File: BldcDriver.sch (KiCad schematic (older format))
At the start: 54 parts, among them J1 Motor Out, J2 DC Jack, J3 STM32_Debug_5pin, Q1 2SK4033, Q2 2SK4033, Q3 2SK4033, Q4 2SK4033, Q5 2SK4033, Q6 2SK4033, U1 IR2101, U2 IR2101, U3 IR2101, U4 NJM78L33SU3, U5 STM32F303K8Tx, X1 12MHz

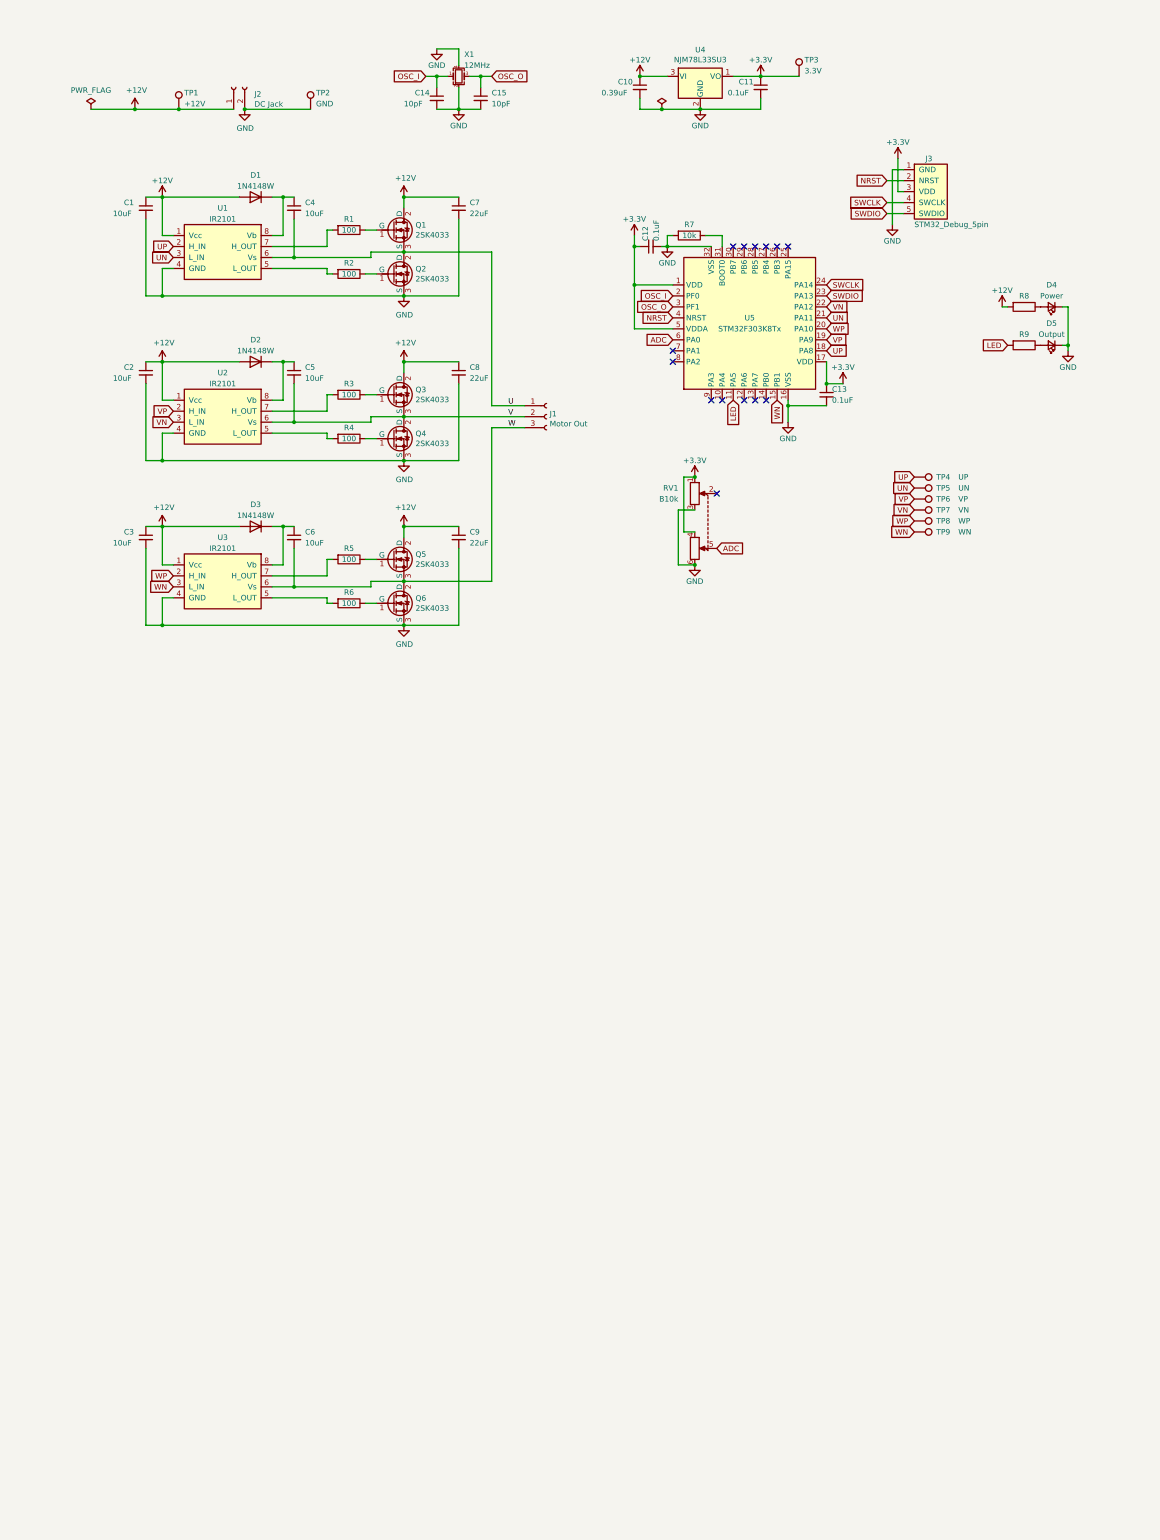
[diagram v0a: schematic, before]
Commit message: 基板 V4.0
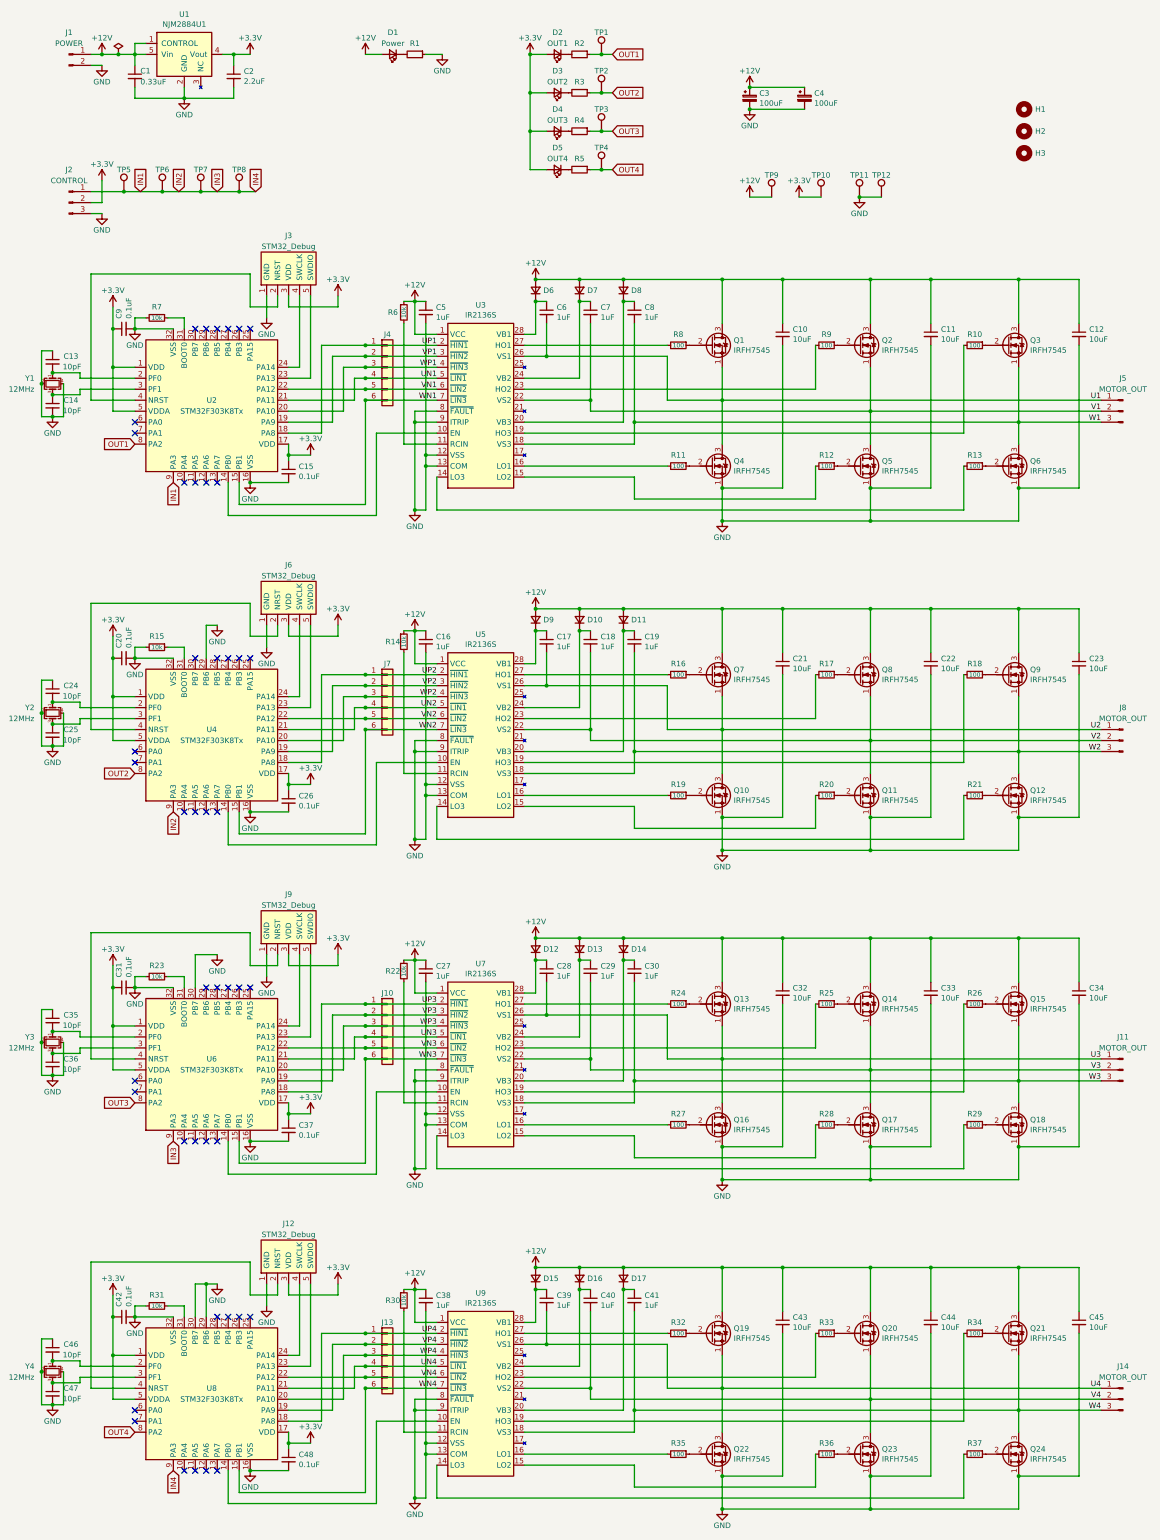
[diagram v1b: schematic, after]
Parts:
- removed C3, C4: 10uF, Capacitor_SMD:C_0603_1608Metric_Pad1.05x0.95mm_HandSolder, symbol Device:C_Small
- removed D1, D2, D3: 1N4148W, Diode_SMD:D_SOD-123, symbol Device:D
- removed J1: Motor Out, Connector_PinSocket_2.54mm:PinSocket_1x03_P2.54mm_Vertical, symbol Connector:Conn_01x03_Female
- removed J2: DC Jack, Connector_PinSocket_2.54mm:PinSocket_1x02_P2.54mm_Vertical, symbol Connector:Conn_01x02_Female
- removed Q1, Q2, Q3, Q4, Q5, Q6: 2SK4033, Package_TO_SOT_THT:TO-220-3_Vertical, symbol BldcDriver:2SK4017
- removed R1, R2, R3, R4, R5, R6: 100, Resistor_SMD:R_0603_1608Metric_Pad1.05x0.95mm_HandSolder, symbol Device:R
- removed R7: 10k, Resistor_SMD:R_0603_1608Metric_Pad1.05x0.95mm_HandSolder, symbol Device:R
- removed R8, R9: R, Resistor_SMD:R_0603_1608Metric_Pad1.05x0.95mm_HandSolder, symbol Device:R
- removed RV1: B10k, Potentiometer_THT:Potentiometer_Alps_RK097_Dual_Horizontal, symbol Device:R_POT_Dual
- removed U1, U2, U3: IR2101, BldcDriver:SOIC-8_3.9x4.9mm_P1.27mm, symbol BldcDriver:IR2101
- removed U4: NJM78L33SU3, Package_TO_SOT_SMD:SOT-89-3, symbol BldcDriver:NJM78L33SU3
- removed U5: STM32F303K8Tx, BldcDriver:LQFP-32_7x7mm_P0.8mm_FusionPCB, symbol BldcDriver:STM32F303K8Tx
- removed X1: 12MHz, BldcDriver:Crystal_SMD_3225-4Pin_3.2x2.5mm_HandSoldering, symbol Device:Crystal_GND24_Small
- added C16, C17, C18, C19, C27, C28, C29, C30, C38, C39, C40, C41: 1uF, BldcDriver:1608Metric, symbol Device:C_Small
- added C20, C26, C31, C37, C42, C48: 0.1uF, BldcDriver:1608Metric, symbol Device:C_Small
- added C21, C22, C23, C32, C33, C34, C43, C44, C45: 10uF, BldcDriver:1608Metric, symbol Device:C_Small
- added C24, C25, C35, C36, C46, C47: 10pF, BldcDriver:1005Metric, symbol Device:C_Small
- added C3, C4: 100uF, BldcDriver:CP_Elec_6.3x7.7, symbol Device:CP_Small
- added D1: Power, BldcDriver:1608Metric, symbol Device:LED_Small
- added D10, D11, D12, D13, D14, D15, D16, D17, D6, D7, D8, D9: 1N4148W, BldcDriver:D_SOD-123, symbol Device:D_Small
- added D2: OUT1, BldcDriver:1608Metric, symbol Device:LED_Small
- added D3: OUT2, BldcDriver:1608Metric, symbol Device:LED_Small
- added H1: MountingHole, BldcDriver:MountingHole_4.3mm_M4, symbol Mechanical:MountingHole
- added H2, H3: MountingHole, BldcDriver:MountingHole_2mm, symbol Mechanical:MountingHole
- added J1: POWER, BldcDriver:JST_XH_S2B-XH-A_1x02_P2.50mm_Horizontal, symbol Connector:Conn_01x02_Male
- added J10, J13, J4, J7: Conn_01x06, BldcDriver:Pin_1x06_P2.54mm, symbol Connector_Generic:Conn_01x06
- added J11, J14, J5, J8: MOTOR_OUT, BldcDriver:JST_XH_S3B-XH-A_1x03_P2.50mm_Horizontal, symbol Connector:Conn_01x03_Male
- added J12, J6, J9: STM32_Debug, BldcDriver:STM32_Debug_5pin, symbol BldcDriver:STM32_Debug_5pin
- added J2: CONTROL, BldcDriver:JST_XH_S3B-XH-A_1x03_P2.50mm_Horizontal, symbol Connector:Conn_01x03_Male
- added Q1, Q10, Q11, Q12, Q13, Q14, Q15, Q16, Q17, Q18, Q19, Q2, Q20, Q21, Q22, Q23, Q24, Q3, Q4, Q5, Q6, Q7, Q8, Q9: IRFH7545, BldcDriver:VSONP-8-1EP_5x6_P1.27mm, symbol Device:Q_NMOS_SGD
- added R1, R2, R3, R4, R5: R, BldcDriver:1608Metric, symbol Device:R_Small
- added R10, R11, R12, R13, R16, R17, R18, R19, R20, R21, R24, R25, R26, R27, R28, R29, R32, R33, R34, R35, R36, R37, R8, R9: 100, BldcDriver:1608Metric, symbol Device:R_Small
- added R14, R15, R22, R23, R30, R31, R6, R7: 10k, BldcDriver:1608Metric, symbol Device:R_Small
- added TP10, TP11, TP12: TestPoint, BldcDriver:TestPoint_THTPad_D1.3mm_Drill0.9mm, symbol Connector:TestPoint
- added U1: NJM2884U1, BldcDriver:SOT-89-5, symbol BldcDriver:NJM2884U1
- added U2, U4, U6, U8: STM32F303K8Tx, BldcDriver:LQFP-32_7x7mm_P0.8mm_FusionPCB, symbol BldcDriver:STM32F303K8Tx
- added U3, U5, U7, U9: IR2136S, BldcDriver:SOIC-28W_7.5x17.9mm_P1.27mm, symbol BldcDriver:IR2136S
- added Y1, Y2, Y3, Y4: 12MHz, BldcDriver:Crystal_SMD_3225-4Pin_3.2x2.5mm_HandSoldering, symbol Device:Crystal_GND24_Small
- C1: value 10uF -> 0.33uF; footprint Capacitor_SMD:C_0603_1608Metric_Pad1.05x0.95mm_HandSolder -> BldcDriver:1608Metric
- C10: value 0.39uF -> 10uF; footprint Capacitor_SMD:C_0603_1608Metric_Pad1.05x0.95mm_HandSolder -> BldcDriver:1608Metric
- C11, C12: value 0.1uF -> 10uF; footprint Capacitor_SMD:C_0603_1608Metric_Pad1.05x0.95mm_HandSolder -> BldcDriver:1608Metric
- C13: value 0.1uF -> 10pF; footprint Capacitor_SMD:C_0603_1608Metric_Pad1.05x0.95mm_HandSolder -> BldcDriver:1005Metric
- C14: footprint BldcDriver:C_0402_1005Metric -> BldcDriver:1005Metric
- C15: value 10pF -> 0.1uF; footprint BldcDriver:C_0402_1005Metric -> BldcDriver:1608Metric
- C2: value 10uF -> 2.2uF; footprint Capacitor_SMD:C_0603_1608Metric_Pad1.05x0.95mm_HandSolder -> BldcDriver:1608Metric
- C5, C6: value 10uF -> 1uF; footprint Capacitor_SMD:C_0603_1608Metric_Pad1.05x0.95mm_HandSolder -> BldcDriver:1608Metric
- C7, C8: value 22uF -> 1uF; footprint Capacitor_SMD:C_1210_3225Metric_Pad1.42x2.65mm_HandSolder -> BldcDriver:1608Metric
- C9: value 22uF -> 0.1uF; footprint Capacitor_SMD:C_1210_3225Metric_Pad1.42x2.65mm_HandSolder -> BldcDriver:1608Metric
- D4: value Power -> OUT3; footprint LED_SMD:LED_0603_1608Metric_Pad1.05x0.95mm_HandSolder -> BldcDriver:1608Metric
- D5: value Output -> OUT4; footprint LED_SMD:LED_0603_1608Metric_Pad1.05x0.95mm_HandSolder -> BldcDriver:1608Metric
- J3: value STM32_Debug_5pin -> STM32_Debug
- TP1: value +12V -> TestPoint; footprint BldcDriver:TestPoint_THTPad_D2.0mm_Drill1.0mm -> BldcDriver:TestPoint_THTPad_D1.3mm_Drill0.9mm
- TP2: value GND -> TestPoint; footprint BldcDriver:TestPoint_THTPad_D2.0mm_Drill1.0mm -> BldcDriver:TestPoint_THTPad_D1.3mm_Drill0.9mm
- TP3: value 3.3V -> TestPoint; footprint BldcDriver:TestPoint_THTPad_D2.0mm_Drill1.0mm -> BldcDriver:TestPoint_THTPad_D1.3mm_Drill0.9mm
- TP4: value UP -> TestPoint; footprint BldcDriver:TestPoint_THTPad_D2.0mm_Drill1.0mm -> BldcDriver:TestPoint_THTPad_D1.3mm_Drill0.9mm
- TP5: value UN -> TestPoint; footprint BldcDriver:TestPoint_THTPad_D2.0mm_Drill1.0mm -> BldcDriver:TestPoint_THTPad_D1.3mm_Drill0.9mm
- TP6: value VP -> TestPoint; footprint BldcDriver:TestPoint_THTPad_D2.0mm_Drill1.0mm -> BldcDriver:TestPoint_THTPad_D1.3mm_Drill0.9mm
- TP7: value VN -> TestPoint; footprint BldcDriver:TestPoint_THTPad_D2.0mm_Drill1.0mm -> BldcDriver:TestPoint_THTPad_D1.3mm_Drill0.9mm
- TP8: value WP -> TestPoint; footprint BldcDriver:TestPoint_THTPad_D2.0mm_Drill1.0mm -> BldcDriver:TestPoint_THTPad_D1.3mm_Drill0.9mm
- TP9: value WN -> TestPoint; footprint BldcDriver:TestPoint_THTPad_D2.0mm_Drill1.0mm -> BldcDriver:TestPoint_THTPad_D1.3mm_Drill0.9mm
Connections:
- net OSC_O is gone; now on net +3V3: C15.1
- net V is gone; now on net GND: C5.2
- net VN is gone; now on net IN1: TP7.1
- net VP is gone; now on net IN1: TP6.1
- net WN is gone; now on net +12V: TP9.1
- net WP is gone; now on net IN1: TP8.1
- net +12V: now also C11.1, C12.1, C5.1, C16.1, C21.1, C22.1, C23.1, C27.1, C3.1, C32.1, C33.1, C34.1, C38.1, C4.1, C43.1, C44.1, C45.1, D1.2 (A), D10.2 (A), D11.2 (A), D12.2 (A), D13.2 (A), D14.2 (A), D15.2 (A), D16.2 (A), D17.2 (A), D6.2 (A), D7.2 (A), D8.2 (A), D9.2 (A), J1.1 (Pin_1), Q1.3 (D), Q13.3 (D), Q14.3 (D), Q15.3 (D), Q19.3 (D), Q2.3 (D), Q20.3 (D), Q21.3 (D), Q3.3 (D), Q7.3 (D), Q8.3 (D), Q9.3 (D), R14.1, R22.1, R30.1, R6.1, U1.1 (CONTROL), U1.5 (Vin), U3.1 (VCC), U5.1 (VCC), U7.1 (VCC), U9.1 (VCC); no longer C2.1, C7.1, C8.1, C9.1, TP1.1
- net +3V3: now also C2.1, C9.1, D4.2 (A), D5.2 (A), C20.1, C26.1, C31.1, C37.1, C42.1, C48.1, D2.2 (A), D3.2 (A), J12.3 (VDD), J2.2 (Pin_2), J6.3 (VDD), J9.3 (VDD), TP10.1, U1.4 (Vout), U2.1 (VDD), U2.17 (VDD), U2.5 (VDDA), U4.1 (VDD), U4.17 (VDD), U4.5 (VDDA), U6.1 (VDD), U6.17 (VDD), U6.5 (VDDA), U8.1 (VDD), U8.17 (VDD), U8.5 (VDDA); no longer C11.1, C12.1, C13.1, TP3.1
- net GND: now also C13.1, C16.2, C20.2, C21.2, C22.2, C23.2, C24.1, C25.2, C26.2, C27.2, C3.2, C31.2, C32.2, C33.2, C34.2, C35.1, C36.2, C37.2, C38.2, C4.2, C42.2, C43.2, C44.2, C45.2, C46.1, C47.2, C48.2, J1.2 (Pin_2), J12.1 (GND), J2.3 (Pin_3), J6.1 (GND), J9.1 (GND), Q10.1 (S), Q11.1 (S), Q12.1 (S), Q16.1 (S), Q17.1 (S), Q18.1 (S), Q22.1 (S), Q23.1 (S), Q24.1 (S), Q4.1 (S), Q5.1 (S), Q6.1 (S), R1.1, R15.2, R23.2, R31.2, R7.2, TP11.1, TP12.1, U1.2 (GND), U2.16 (VSS), U2.32 (VSS), U3.12 (VSS), U3.13 (COM), U3.8 (~FAULT), U3.9 (ITRIP), U4.16 (VSS), U4.29 (PB6), U4.32 (VSS), U5.12 (VSS), U5.13 (COM), U5.8 (~FAULT), U5.9 (ITRIP), U6.16 (VSS), U6.30 (PB7), U6.32 (VSS), U7.12 (VSS), U7.13 (COM), U7.8 (~FAULT), U7.9 (ITRIP), U8.16 (VSS), U8.29 (PB6), U8.30 (PB7), U8.32 (VSS), U9.12 (VSS), U9.13 (COM), U9.8 (~FAULT), U9.9 (ITRIP), Y1.2, Y1.4, Y2.2, Y2.4, Y3.2, Y3.4, Y4.2, Y4.4; no longer C13.2, C7.2, C8.2, D4.1 (K), D5.1 (K), TP2.1
- net at C6.1: now also D6.1 (K), U3.28 (VB1)
- net NRST: no longer names the net of J3.2 (NRST)
- net NRST: now also U2.4 (NRST)
- net OSC_I: no longer names the net of C14.1
- net OSC_I: now also U2.3 (PF1), Y1.3
- net SWCLK: no longer names the net of J3.4 (SWCLK)
- net SWCLK: now also U2.24 (PA14)
- net SWDIO: no longer names the net of J3.5 (SWDIO)
- net SWDIO: now also U2.23 (PA13)
- net UN renamed IN1
- net IN1: now also J2.1 (Pin_1), U2.9 (PA3), U4.9 (PA3), U6.9 (PA3), U8.9 (PA3)
- net UP renamed OUT4
- net OUT4: now also R5.1, U8.8 (PA2)
- net W renamed U1
- net U1: now also J5.1 (Pin_1), Q1.1 (S), Q4.3 (D), U3.26 (VS1)
- new net: U2.14 (PB0), U3.10 (EN)
- new net: R6.2, U3.11 (RCIN)
- new net: R13.2, U3.14 (LO3)
- new net: R12.2, U3.15 (LO2)
- new net: R11.2, U3.16 (LO1)
- new net: R10.2, U3.19 (HO3)
- new net: C8.1, D8.1 (K), U3.20 (VB3)
- new net: R9.2, U3.23 (HO2)
- new net: C7.1, D7.1 (K), U3.24 (VB2)
- new net: R8.2, U3.27 (HO1)
- new net: C13.2, U2.2 (PF0), Y1.1
- new net: R7.1, U2.31 (BOOT0)
- new net: Q1.2 (G), R8.1
- new net: Q4.2 (G), R11.1
- new net: Q2.2 (G), R9.1
- new net: Q5.2 (G), R12.1
- new net: Q3.2 (G), R10.1
- new net: Q6.2 (G), R13.1
- new net: U4.14 (PB0), U5.10 (EN)
- new net: R14.2, U5.11 (RCIN)
- new net: R21.2, U5.14 (LO3)
- new net: R20.2, U5.15 (LO2)
- new net: R19.2, U5.16 (LO1)
- new net: R18.2, U5.19 (HO3)
- new net: C19.1, D11.1 (K), U5.20 (VB3)
- new net: R17.2, U5.23 (HO2)
- new net: C18.1, D10.1 (K), U5.24 (VB2)
- new net: R16.2, U5.27 (HO1)
- new net: C17.1, D9.1 (K), U5.28 (VB1)
- new net: C24.2, U4.2 (PF0), Y2.1
- new net: J6.5 (SWDIO), U4.23 (PA13)
- new net: J6.4 (SWCLK), U4.24 (PA14)
- new net: C25.1, U4.3 (PF1), Y2.3
- new net: R15.1, U4.31 (BOOT0)
- new net: J6.2 (NRST), U4.4 (NRST)
- new net: Q7.2 (G), R16.1
- new net: Q10.2 (G), R19.1
- new net: Q8.2 (G), R17.1
- new net: Q11.2 (G), R20.1
- new net: Q9.2 (G), R18.1
- new net: Q12.2 (G), R21.1
- new net: U6.14 (PB0), U7.10 (EN)
- new net: R22.2, U7.11 (RCIN)
- new net: R29.2, U7.14 (LO3)
- new net: R28.2, U7.15 (LO2)
- new net: R27.2, U7.16 (LO1)
- new net: R26.2, U7.19 (HO3)
- new net: C30.1, D14.1 (K), U7.20 (VB3)
- new net: R25.2, U7.23 (HO2)
- new net: C29.1, D13.1 (K), U7.24 (VB2)
- new net: R24.2, U7.27 (HO1)
- new net: C28.1, D12.1 (K), U7.28 (VB1)
- new net: C35.2, U6.2 (PF0), Y3.1
- new net: J9.5 (SWDIO), U6.23 (PA13)
- new net: J9.4 (SWCLK), U6.24 (PA14)
- new net: C36.1, U6.3 (PF1), Y3.3
- new net: R23.1, U6.31 (BOOT0)
- new net: J9.2 (NRST), U6.4 (NRST)
- new net: Q13.2 (G), R24.1
- new net: Q16.2 (G), R27.1
- new net: Q14.2 (G), R25.1
- new net: Q17.2 (G), R28.1
- new net: Q15.2 (G), R26.1
- new net: Q18.2 (G), R29.1
- new net: U8.14 (PB0), U9.10 (EN)
- new net: R30.2, U9.11 (RCIN)
- new net: R37.2, U9.14 (LO3)
- new net: R36.2, U9.15 (LO2)
- new net: R35.2, U9.16 (LO1)
- new net: R34.2, U9.19 (HO3)
- new net: C41.1, D17.1 (K), U9.20 (VB3)
- new net: R33.2, U9.23 (HO2)
- new net: C40.1, D16.1 (K), U9.24 (VB2)
- new net: R32.2, U9.27 (HO1)
- new net: C39.1, D15.1 (K), U9.28 (VB1)
- new net: C46.2, U8.2 (PF0), Y4.1
- new net: J12.5 (SWDIO), U8.23 (PA13)
- new net: J12.4 (SWCLK), U8.24 (PA14)
- new net: C47.1, U8.3 (PF1), Y4.3
- new net: R31.1, U8.31 (BOOT0)
- new net: J12.2 (NRST), U8.4 (NRST)
- new net: Q19.2 (G), R32.1
- new net: Q22.2 (G), R35.1
- new net: Q20.2 (G), R33.1
- new net: Q23.2 (G), R36.1
- new net: Q21.2 (G), R34.1
- new net: Q24.2 (G), R37.1
- new net: D3.1 (K), R3.2
- new net: D4.1 (K), R4.2
- new net: D5.1 (K), R5.2
- new net: D1.1 (K), R1.2
- new net: D2.1 (K), R2.2
- new net OUT1: R2.1, TP1.1, U2.8 (PA2)
- new net OUT2: R3.1, TP2.1, U4.8 (PA2)
- new net OUT3: R4.1, TP3.1, U6.8 (PA2)
- new net U2: C17.2, J8.1 (Pin_1), Q10.3 (D), Q7.1 (S), U5.26 (VS1)
- new net U3: C28.2, J11.1 (Pin_1), Q13.1 (S), Q16.3 (D), U7.26 (VS1)
- new net U4: C39.2, J14.1 (Pin_1), Q19.1 (S), Q22.3 (D), U9.26 (VS1)
- new net UN1: J4.4 (Pin_4), U2.21 (PA11), U3.5 (~LIN1)
- new net UN2: J7.4 (Pin_4), U4.21 (PA11), U5.5 (~LIN1)
- new net UN3: J10.4 (Pin_4), U6.21 (PA11), U7.5 (~LIN1)
- new net UN4: J13.4 (Pin_4), U8.21 (PA11), U9.5 (~LIN1)
- new net UP1: J4.1 (Pin_1), U2.18 (PA8), U3.2 (~HIN1)
- new net UP2: J7.1 (Pin_1), U4.18 (PA8), U5.2 (~HIN1)
- new net UP3: J10.1 (Pin_1), U6.18 (PA8), U7.2 (~HIN1)
- new net UP4: J13.1 (Pin_1), U8.18 (PA8), U9.2 (~HIN1)
- new net V1: C7.2, J5.2 (Pin_2), Q2.1 (S), Q5.3 (D), U3.22 (VS2)
- new net V2: C18.2, J8.2 (Pin_2), Q11.3 (D), Q8.1 (S), U5.22 (VS2)
- new net V3: C29.2, J11.2 (Pin_2), Q14.1 (S), Q17.3 (D), U7.22 (VS2)
- new net V4: C40.2, J14.2 (Pin_2), Q20.1 (S), Q23.3 (D), U9.22 (VS2)
- new net VN1: J4.5 (Pin_5), U2.22 (PA12), U3.6 (~LIN2)
- new net VN2: J7.5 (Pin_5), U4.22 (PA12), U5.6 (~LIN2)
- new net VN3: J10.5 (Pin_5), U6.22 (PA12), U7.6 (~LIN2)
- new net VN4: J13.5 (Pin_5), U8.22 (PA12), U9.6 (~LIN2)
- new net VP1: J4.2 (Pin_2), U2.19 (PA9), U3.3 (~HIN2)
- new net VP2: J7.2 (Pin_2), U4.19 (PA9), U5.3 (~HIN2)
- new net VP3: J10.2 (Pin_2), U6.19 (PA9), U7.3 (~HIN2)
- new net VP4: J13.2 (Pin_2), U8.19 (PA9), U9.3 (~HIN2)
- new net W1: C8.2, J5.3 (Pin_3), Q3.1 (S), Q6.3 (D), U3.18 (VS3)
- new net W2: C19.2, J8.3 (Pin_3), Q12.3 (D), Q9.1 (S), U5.18 (VS3)
- new net W3: C30.2, J11.3 (Pin_3), Q15.1 (S), Q18.3 (D), U7.18 (VS3)
- new net W4: C41.2, J14.3 (Pin_3), Q21.1 (S), Q24.3 (D), U9.18 (VS3)
- new net WN1: J4.6 (Pin_6), U2.15 (PB1), U3.7 (~LIN3)
- new net WN2: J7.6 (Pin_6), U4.15 (PB1), U5.7 (~LIN3)
- new net WN3: J10.6 (Pin_6), U6.15 (PB1), U7.7 (~LIN3)
- new net WN4: J13.6 (Pin_6), U8.15 (PB1), U9.7 (~LIN3)
- new net WP1: J4.3 (Pin_3), U2.20 (PA10), U3.4 (~HIN3)
- new net WP2: J7.3 (Pin_3), U4.20 (PA10), U5.4 (~HIN3)
- new net WP3: J10.3 (Pin_3), U6.20 (PA10), U7.4 (~HIN3)
- new net WP4: J13.3 (Pin_3), U8.20 (PA10), U9.4 (~HIN3)
- no-connect marks 14 -> 44
